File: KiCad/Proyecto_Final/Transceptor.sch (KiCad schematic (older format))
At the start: 40 parts, among them U1 hackrf_MAX2837

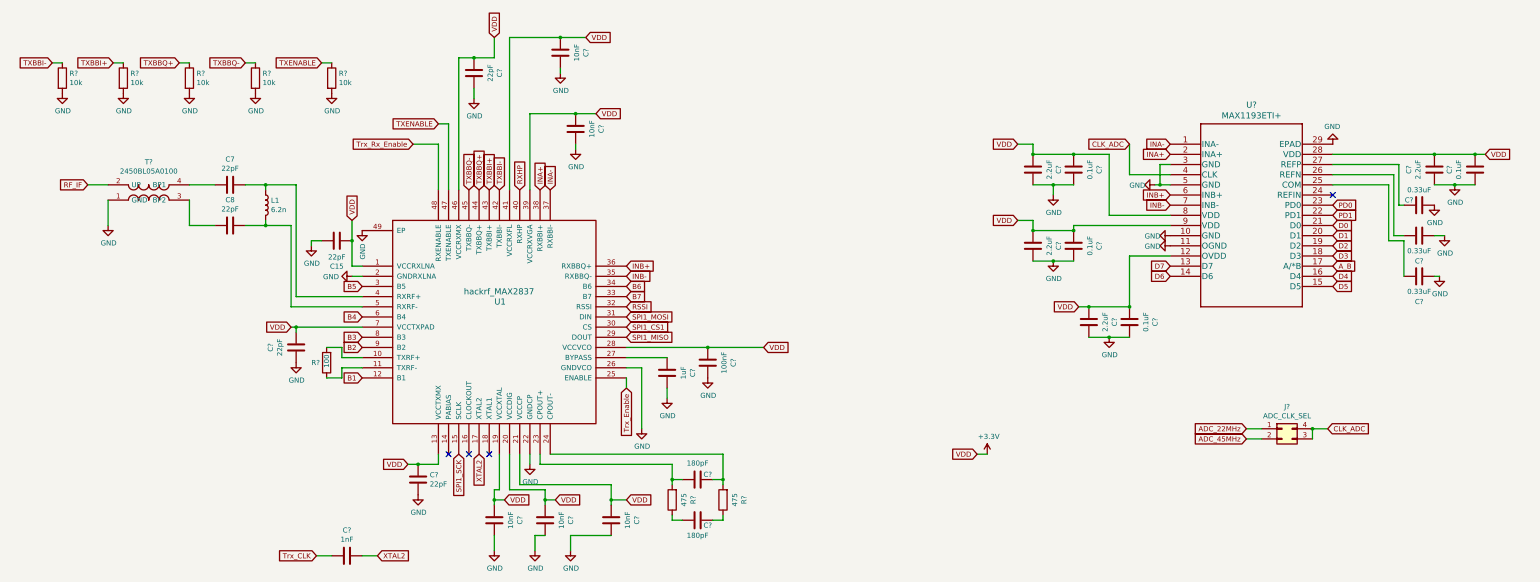
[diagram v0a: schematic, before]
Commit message: Esquematico terminado con test points.
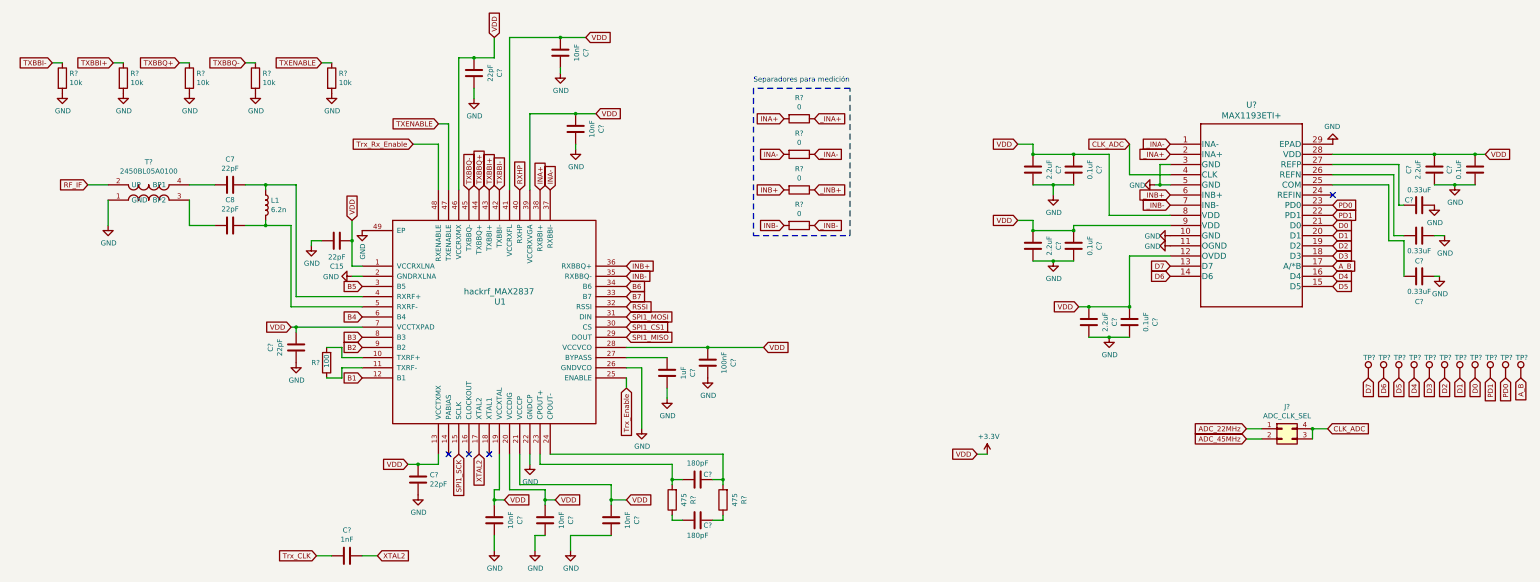
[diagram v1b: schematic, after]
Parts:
- added R? (x4): 0, symbol Device:R
- added TP? (x11): TestPoint, symbol Connector:TestPoint
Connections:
- net A_B: now also TP?.1
- net D0: now also TP?.1
- net D1: now also TP?.1
- net D2: now also TP?.1
- net D3: now also TP?.1
- net D4: now also TP?.1
- net D5: now also TP?.1
- net D6: now also TP?.1
- net D7: now also TP?.1
- net INA+: now also R?.2; no longer U?.2 (INA+)
- net INA-: now also R?.2; no longer U?.1 (INA-)
- net INB+: now also R?.2; no longer U?.6 (INB+)
- net INB-: now also R?.2; no longer U?.7 (INB-)
- net PD0: now also TP?.1
- net PD1: now also TP?.1
- new net _INA+: R?.1, U?.2 (INA+)
- new net _INA-: R?.1, U?.1 (INA-)
- new net _INB+: R?.1, U?.6 (INB+)
- new net _INB-: R?.1, U?.7 (INB-)
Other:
- note added: "Separadores para medición"
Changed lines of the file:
@@
 Text GLabel 6950 3250 2    50   Input ~ 0
 INB-
-Text GLabel 12300 1950 0    50   Input ~ 0
-INA-
-Text GLabel 12300 2050 0    50   Input ~ 0
-INA+
-Text GLabel 12300 2550 0    50   Input ~ 0
-INB-
-Text GLabel 12300 2450 0    50   Input ~ 0
-INB+
 Wire Wire Line
 	10950 1950 10950 2050
@@
 Wire Wire Line
 	13050 4850 13200 4850
+$Comp
+L Device:R R?
+U 1 1 60791BA0
+P 8650 1700
+F 0 "R?" V 8443 1700 50  0000 C CNN
+F 1 "0" V 8534 1700 50  0000 C CNN
+F 2 "" V 8580 1700 50  0001 C CNN
+F 3 "~" H 8650 1700 50  0001 C CNN
+	1    8650 1700
+	0    1    1    0
+$EndComp
+$Comp
+L Device:R R?
+U 1 1 60798900
+P 8650 2050
+F 0 "R?" V 8443 2050 50  0000 C CNN
+F 1 "0" V 8534 2050 50  0000 C CNN
+F 2 "" V 8580 2050 50  0001 C CNN
+F 3 "~" H 8650 2050 50  0001 C CNN
+	1    8650 2050
+	0    1    1    0
+$EndComp
+$Comp
+L Device:R R?
+U 1 1 60798B8E
+P 8650 2400
+F 0 "R?" V 8443 2400 50  0000 C CNN
+F 1 "0" V 8534 2400 50  0000 C CNN
+F 2 "" V 8580 2400 50  0001 C CNN
+F 3 "~" H 8650 2400 50  0001 C CNN
+	1    8650 2400
+	0    1    1    0
+$EndComp
+$Comp
+L Device:R R?
+U 1 1 60798F18
+P 8650 2750
+F 0 "R?" V 8443 2750 50  0000 C CNN
+F 1 "0" V 8534 2750 50  0000 C CNN
+F 2 "" V 8580 2750 50  0001 C CNN
+F 3 "~" H 8650 2750 50  0001 C CNN
+	1    8650 2750
+	0    1    1    0
+$EndComp
+Text GLabel 8500 1700 0    50   Input ~ 0
+INA+
+Text GLabel 8500 2050 0    50   Input ~ 0
+INA-
+Text GLabel 8500 2400 0    50   Input ~ 0
+INB+
+Text GLabel 8500 2750 0    50   Input ~ 0
+INB-
+Text GLabel 8800 1700 2    50   Input ~ 0
+_INA+
+Text GLabel 8800 2050 2    50   Input ~ 0
+_INA-
+Text GLabel 8800 2400 2    50   Input ~ 0
+_INB+
+Text GLabel 8800 2750 2    50   Input ~ 0
+_INB-
+Text GLabel 12300 2050 0    50   Input ~ 0
+_INA+
+Text GLabel 12300 1950 0    50   Input ~ 0
+_INA-
+Text GLabel 12300 2450 0    50   Input ~ 0
+_INB+
+Text GLabel 12300 2550 0    50   Input ~ 0
+_INB-
+Wire Notes Line
+	8200 1400 8200 2850
+Wire Notes Line
+	8200 2850 9150 2850
+Wire Notes Line
+	9150 2850 9150 1400
+Wire Notes Line
+	9150 1400 8200 1400
+Text Notes 8200 1350 0    50   ~ 0
+Separadores para medición
+Text GLabel 14550 4250 3    50   Input ~ 0
+D5
+Text GLabel 14700 4250 3    50   Input ~ 0
+D4
+Text GLabel 15750 4250 3    50   Input ~ 0
+A_B
+Text GLabel 14850 4250 3    50   Input ~ 0
+D3
+Text GLabel 15000 4250 3    50   Input ~ 0
+D2
+Text GLabel 15150 4250 3    50   Input ~ 0
+D1
+Text GLabel 15300 4250 3    50   Input ~ 0
+D0
+Text GLabel 15450 4250 3    50   Input ~ 0
+PD1
+Text GLabel 15600 4250 3    50   Input ~ 0
+PD0
+$Comp
+L Connector:TestPoint TP?
+U 1 1 607AE5A5
+P 14550 4250
+F 0 "TP?" H 14500 4450 50  0000 L CNN
+F 1 "TestPoint" H 14350 4600 50  0001 L CNN
+F 2 "" H 14750 4250 50  0001 C CNN
+F 3 "~" H 14750 4250 50  0001 C CNN
+	1    14550 4250
+	1    0    0    -1
+$EndComp
+$Comp
+L Connector:TestPoint TP?
+U 1 1 607C1A8B
+P 14700 4250
+F 0 "TP?" H 14650 4450 50  0000 L CNN
+F 1 "TestPoint" H 14500 4600 50  0001 L CNN
+F 2 "" H 14900 4250 50  0001 C CNN
+F 3 "~" H 14900 4250 50  0001 C CNN
+	1    14700 4250
+	1    0    0    -1
+$EndComp
+$Comp
+L Connector:TestPoint TP?
+U 1 1 607DFB6E
+P 15750 4250
+F 0 "TP?" H 15700 4450 50  0000 L CNN
+F 1 "TestPoint" H 15550 4600 50  0001 L CNN
+F 2 "" H 15950 4250 50  0001 C CNN
+F 3 "~" H 15950 4250 50  0001 C CNN
+	1    15750 4250
+	1    0    0    -1
+$EndComp
+$Comp
+L Connector:TestPoint TP?
+U 1 1 607DFE0C
+P 14850 4250
+F 0 "TP?" H 14800 4450 50  0000 L CNN
+F 1 "TestPoint" H 14650 4600 50  0001 L CNN
+F 2 "" H 15050 4250 50  0001 C CNN
+F 3 "~" H 15050 4250 50  0001 C CNN
+	1    14850 4250
+	1    0    0    -1
+$EndComp
+$Comp
+L Connector:TestPoint TP?
+U 1 1 607DFFDB
+P 15000 4250
+F 0 "TP?" H 14950 4450 50  0000 L CNN
+F 1 "TestPoint" H 14800 4600 50  0001 L CNN
+F 2 "" H 15200 4250 50  0001 C CNN
+F 3 "~" H 15200 4250 50  0001 C CNN
+	1    15000 4250
+	1    0    0    -1
+$EndComp
+$Comp
+L Connector:TestPoint TP?
+U 1 1 607E00F5
+P 15150 4250
+F 0 "TP?" H 15100 4450 50  0000 L CNN
+F 1 "TestPoint" H 14950 4600 50  0001 L CNN
+F 2 "" H 15350 4250 50  0001 C CNN
+F 3 "~" H 15350 4250 50  0001 C CNN
+	1    15150 4250
+	1    0    0    -1
+$EndComp
+$Comp
+L Connector:TestPoint TP?
+U 1 1 607E0392
+P 15300 4250
+F 0 "TP?" H 15250 4450 50  0000 L CNN
+F 1 "TestPoint" H 15100 4600 50  0001 L CNN
+F 2 "" H 15500 4250 50  0001 C CNN
+F 3 "~" H 15500 4250 50  0001 C CNN
+	1    15300 4250
+	1    0    0    -1
+$EndComp
+$Comp
+L Connector:TestPoint TP?
+U 1 1 607E0698
+P 15450 4250
+F 0 "TP?" H 15400 4450 50  0000 L CNN
+F 1 "TestPoint" H 15250 4600 50  0001 L CNN
+F 2 "" H 15650 4250 50  0001 C CNN
+F 3 "~" H 15650 4250 50  0001 C CNN
+	1    15450 4250
+	1    0    0    -1
+$EndComp
+$Comp
+L Connector:TestPoint TP?
+U 1 1 607E08DA
+P 15600 4250
+F 0 "TP?" H 15550 4450 50  0000 L CNN
+F 1 "TestPoint" H 15400 4600 50  0001 L CNN
+F 2 "" H 15800 4250 50  0001 C CNN
+F 3 "~" H 15800 4250 50  0001 C CNN
+	1    15600 4250
+	1    0    0    -1
+$EndComp
+Text GLabel 14250 4250 3    50   Input ~ 0
+D7
+Text GLabel 14400 4250 3    50   Input ~ 0
+D6
+$Comp
+L Connector:TestPoint TP?
+U 1 1 607E6856
+P 14400 4250
+F 0 "TP?" H 14350 4450 50  0000 L CNN
+F 1 "TestPoint" H 14200 4600 50  0001 L CNN
+F 2 "" H 14600 4250 50  0001 C CNN
+F 3 "~" H 14600 4250 50  0001 C CNN
+	1    14400 4250
+	1    0    0    -1
+$EndComp
+$Comp
+L Connector:TestPoint TP?
+U 1 1 607E6ACC
+P 14250 4250
+F 0 "TP?" H 14200 4450 50  0000 L CNN
+F 1 "TestPoint" H 14050 4600 50  0001 L CNN
+F 2 "" H 14450 4250 50  0001 C CNN
+F 3 "~" H 14450 4250 50  0001 C CNN
+	1    14250 4250
+	1    0    0    -1
+$EndComp
 $EndSCHEMATC
